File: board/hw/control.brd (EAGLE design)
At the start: 100 x 80 mm, 33 parts, among them T1 pn2222a, T2 pn2222a, T3 pn2222a, T4 pn2222a, T5 pn2222a, T6 pn2222a, T7 pn2222a, T8 pn2222a

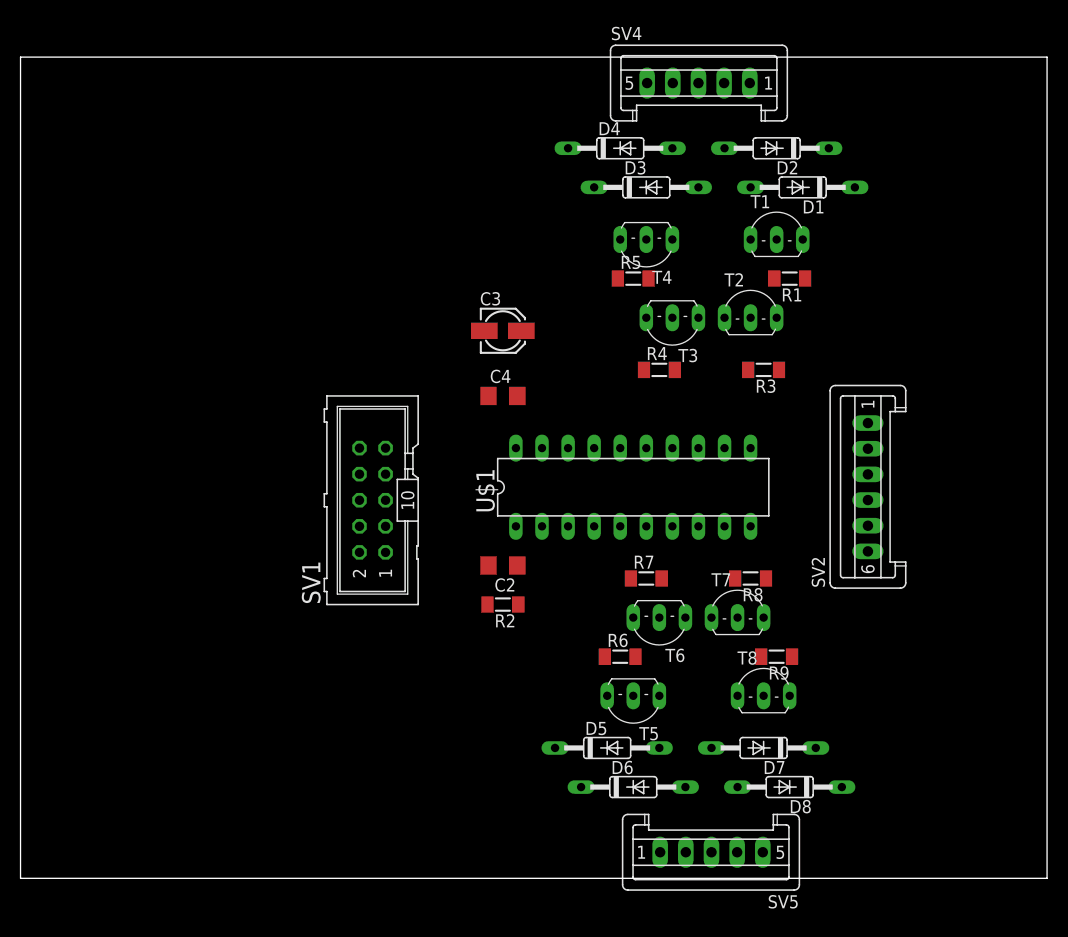
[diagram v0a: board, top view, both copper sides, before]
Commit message: single-layer routing completed (yay)
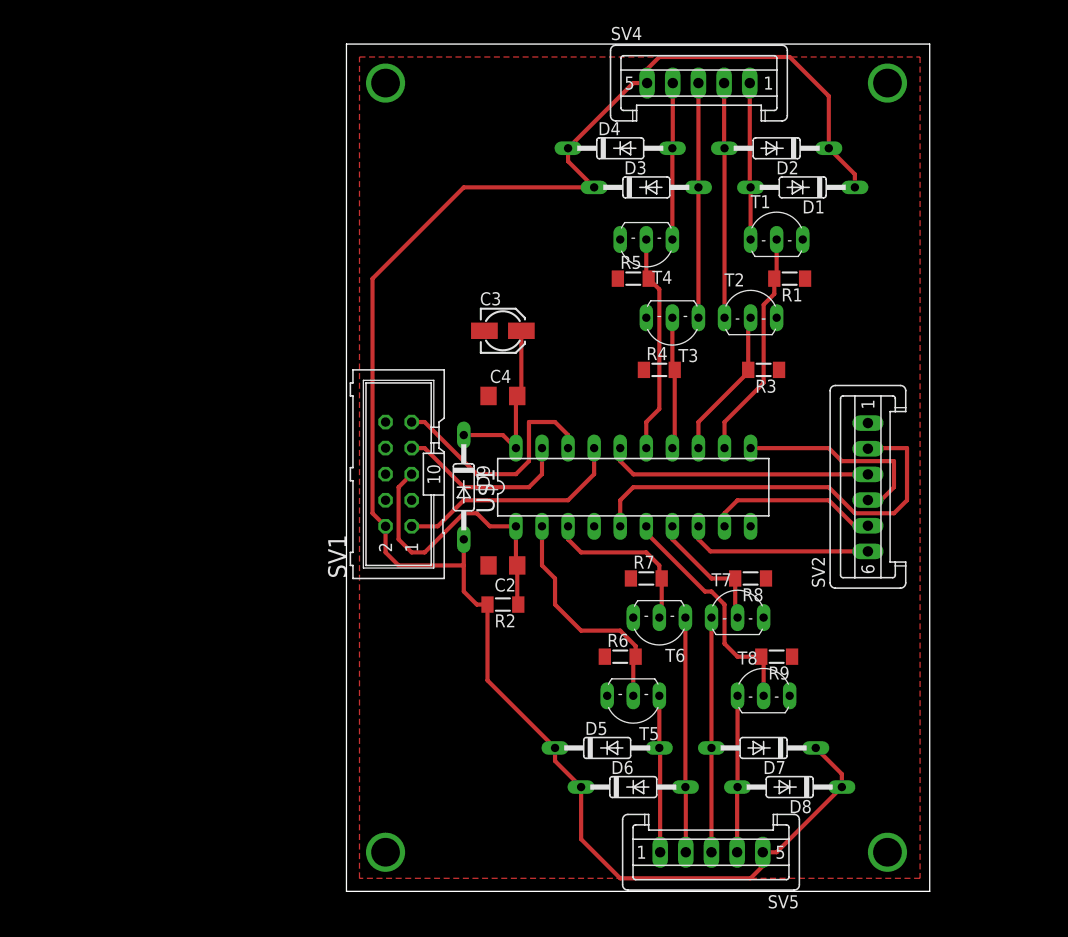
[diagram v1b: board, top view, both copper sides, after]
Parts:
- added D9: 1N4446, diode:DO35-10
- moved SV1 3.59 mm to (36.8, 39.4)
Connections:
- new net N$26: C3.+, C4.2, D9.C, U$1.20
- net +5V: now also D9.A; no longer C3.+, C4.2, U$1.20
- net N$11: now also U$1.13; no longer U$1.14
- net N$13: now also U$1.14; no longer U$1.13
- net N$15: now also U$1.15; no longer U$1.12
- net N$18: now also U$1.6; no longer U$1.7
- net N$6: now also U$1.7; no longer U$1.6
- net N$9: now also U$1.12; no longer U$1.15
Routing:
- net +5V: track 0.00 -> 177.7 mm
- net N$25: track 0.00 -> 41.5 mm
- net N$16: track 0.00 -> 28.7 mm
- net N$24: track 0.00 -> 25.9 mm
- net N$20: track 0.00 -> 23.5 mm
- net N$18: track 0.00 -> 23.0 mm
- net N$21: track 0.00 -> 22.9 mm
- net N$10: track 0.00 -> 22.9 mm
- net N$5: track 0.00 -> 22.9 mm
- net N$12: track 0.00 -> 22.9 mm
- net N$2: track 0.00 -> 22.6 mm
- net N$9: track 0.00 -> 22.4 mm
- net N$17: track 0.00 -> 22.4 mm
- net N$15: track 0.00 -> 21.4 mm
- net N$23: track 0.00 -> 20.1 mm
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- added copper zone on layer 1, net 0V
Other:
- board size 100 x 80 mm -> 56.8 x 82.5 mm
